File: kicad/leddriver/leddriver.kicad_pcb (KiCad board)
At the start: 2 copper layers, 37.8 x 19.3 mm, 7 parts, among them J1 Conn_01x02_Male, J2 Conn_01x01_Male, U1 TLC555xP

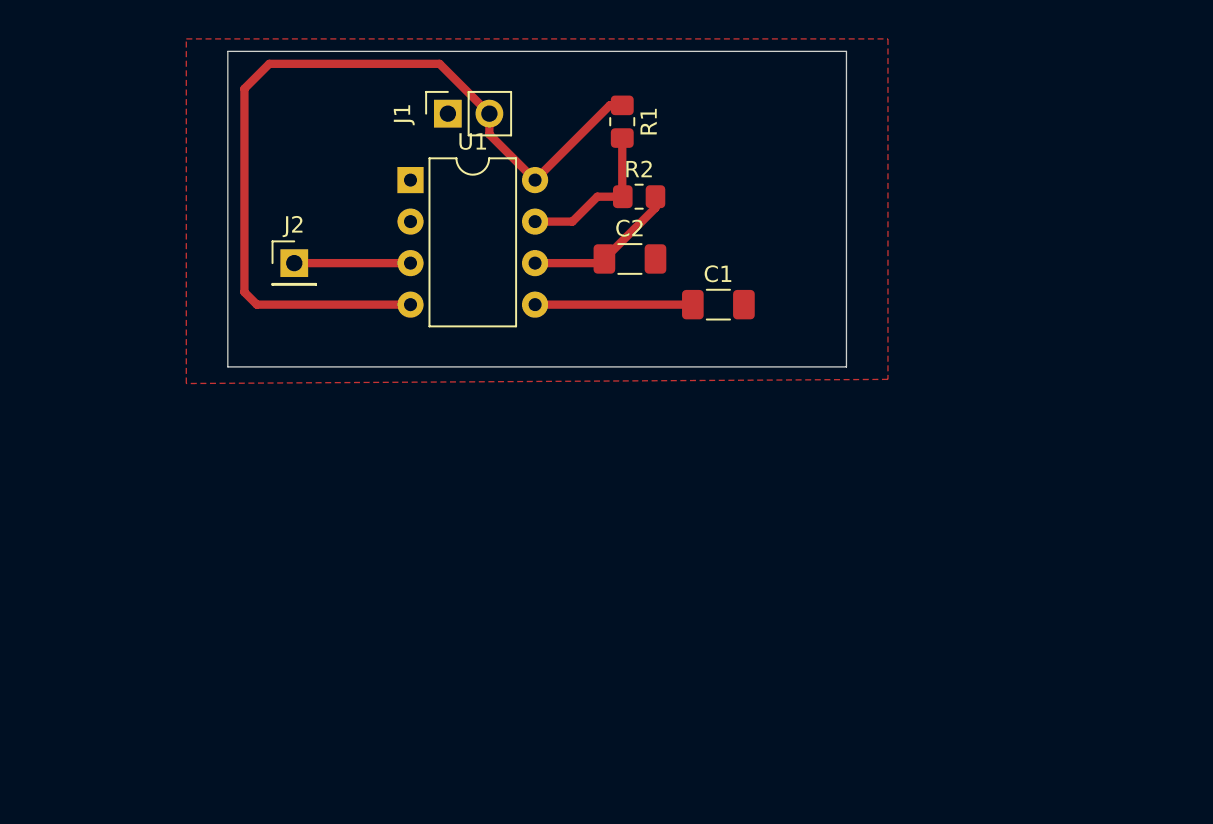
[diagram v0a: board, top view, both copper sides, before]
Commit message: Add new code
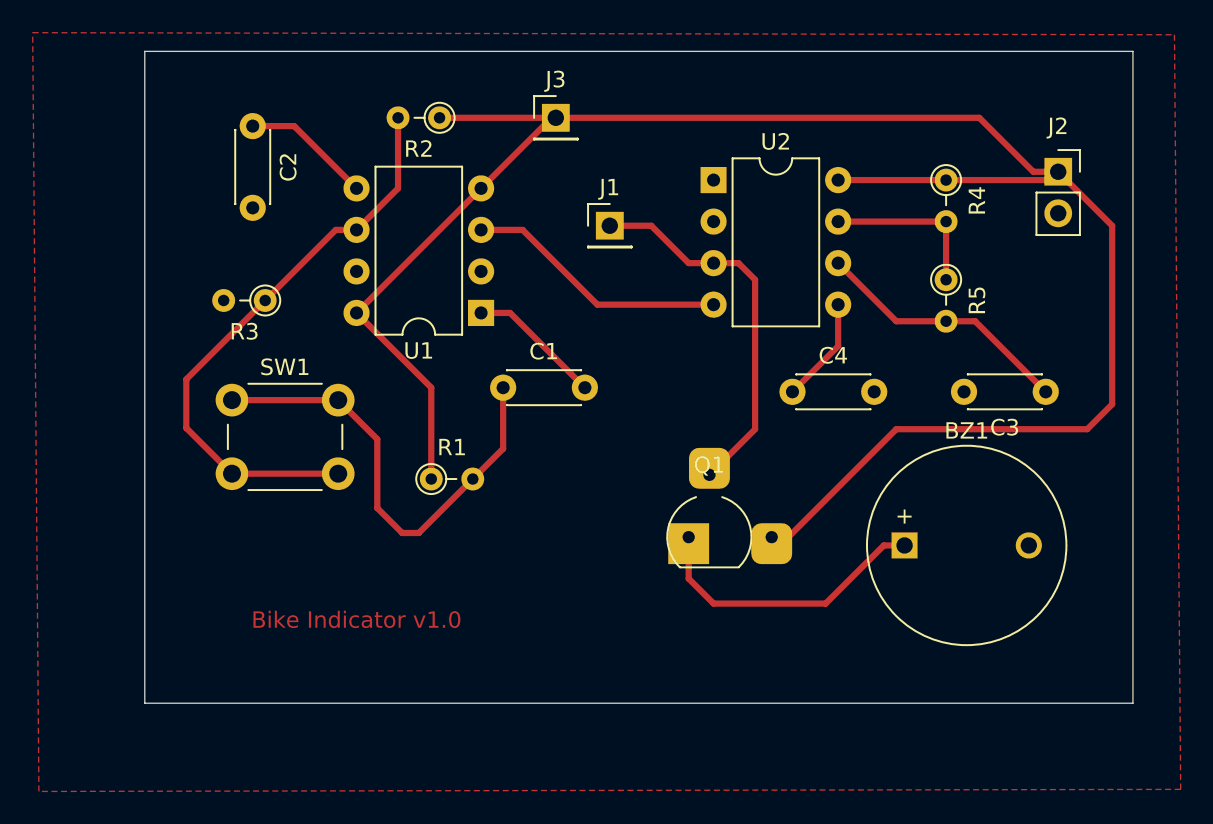
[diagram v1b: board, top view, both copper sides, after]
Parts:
- added BZ1: Buzzer, Buzzer_Beeper:MagneticBuzzer_ProSignal_ABI-010-RC, F.Cu at (165.9, 99.6)
- added C3: 4.7uF, Capacitor_THT:C_Disc_D4.3mm_W1.9mm_P5.00mm, F.Cu at (174.5, 90.2)
- added C4: .01uF, Capacitor_THT:C_Disc_D4.3mm_W1.9mm_P5.00mm, F.Cu at (159.0, 90.2)
- added J3: Conn_01x01_Male, Connector_PinHeader_2.54mm:PinHeader_1x01_P2.54mm_Vertical, F.Cu at (144.5, 73.4)
- added Q1: 2N3904, leddriver:TO-92_HandSolder_Large_Pad, F.Cu at (152.7, 99.1)
- added R3: 68k, Resistor_THT:R_Axial_DIN0204_L3.6mm_D1.6mm_P2.54mm_Vertical, F.Cu at (126.7, 84.6)
- added R4: 1k, Resistor_THT:R_Axial_DIN0204_L3.6mm_D1.6mm_P2.54mm_Vertical, F.Cu at (168.4, 77.2)
- added R5: 68k, Resistor_THT:R_Axial_DIN0204_L3.6mm_D1.6mm_P2.54mm_Vertical, F.Cu at (168.4, 83.3)
- added SW1: SW_Push, Button_Switch_THT:SW_PUSH_6mm_H5mm, F.Cu at (124.7, 90.7)
- added U2: TLC555xP, Package_DIP:DIP-8_W7.62mm, F.Cu at (154.2, 77.2)
- C1: value 0.01uF -> 1uF; footprint Capacitor_SMD:C_1206_3216Metric_Pad1.33x1.80mm_HandSolder -> Capacitor_THT:C_Disc_D4.3mm_W1.9mm_P5.00mm
- C2: value 10uF -> .01uF; footprint Capacitor_SMD:C_1206_3216Metric_Pad1.33x1.80mm_HandSolder -> Capacitor_THT:C_Disc_D4.3mm_W1.9mm_P5.00mm
- J1: value Conn_01x02_Male -> Conn_01x01_Male; footprint Connector_PinSocket_2.54mm:PinSocket_1x02_P2.54mm_Vertical -> Connector_PinHeader_2.54mm:PinHeader_1x01_P2.54mm_Vertical
- J2: value Conn_01x01_Male -> Conn_01x02_Male; footprint Connector_PinHeader_2.54mm:PinHeader_1x01_P2.54mm_Vertical -> Connector_PinSocket_2.54mm:PinSocket_1x02_P2.54mm_Vertical
- R1, R2: footprint Resistor_SMD:R_0805_2012Metric_Pad1.20x1.40mm_HandSolder -> Resistor_THT:R_Axial_DIN0204_L3.6mm_D1.6mm_P2.54mm_Vertical
- moved J2 47.1 mm to (175.3, 76.7)
- moved R1 24.8 mm to (136.9, 95.5), turned to 0 degrees
- moved C2 24.5 mm to (126.0, 73.9), turned to 270 degrees
- moved C1 14.1 mm to (141.3, 89.9)
- moved R2 13.1 mm to (137.4, 73.4), turned to 180 degrees
- moved J1 12.0 mm to (147.8, 80.0), turned to 0 degrees
- moved U1 9.20 mm to (140.0, 85.3), turned to 180 degrees
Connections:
- J1 pad 1: GND -> OUT
- J2 pad 1: Net-(J2-Pad1) -> VCC
- R1 pad 2: Net-(R1-Pad2) -> Net-(C1-Pad1)
- R2 pad 1: Net-(R1-Pad2) -> VCC
- R2 pad 2: Net-(C2-Pad1) -> Net-(R2-Pad2)
- U1 pad 2: Net-(C2-Pad1) -> Net-(R2-Pad2)
- U1 pad 3: Net-(J2-Pad1) -> OUT1
- U1 pad 5: Net-(C1-Pad1) -> Net-(C2-Pad1)
- U1 pad 6: Net-(C2-Pad1) -> Net-(R2-Pad2)
- U1 pad 7: Net-(R1-Pad2) -> (no net)
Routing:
- net VCC: track 52.3 -> 122.5 mm
- net Net-(R2-Pad2): track 0.00 -> 35.5 mm
- net OUT: track 0.00 -> 23.4 mm
- net Net-(C1-Pad1): track 9.65 -> 28.3 mm
- net Net-(BZ1-Pad1): track 0.00 -> 18.1 mm
- net OUT1: track 0.00 -> 16.1 mm
- net Net-(C3-Pad1): track 0.00 -> 16.0 mm
- net Net-(R4-Pad2): track 0.00 -> 10.2 mm
- net Net-(R1-Pad2): track 9.60 -> 0.00 mm
- net GND: track 0.00 -> 8.24 mm
- net Net-(J2-Pad1): track 7.11 -> 0.00 mm
- net Net-(C4-Pad1): track 0.00 -> 6.49 mm
- net Net-(C2-Pad1): track 9.45 -> 7.93 mm
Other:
- board size 37.8 x 19.3 mm -> 60.5 x 39.9 mm
- board text added: "Bike Indicator v1.0"
